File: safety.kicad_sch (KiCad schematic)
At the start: 23 parts, among them J5 Screw_Terminal_01x02, J7 Screw_Terminal_01x02, Q4 BSS138, SW1 SW_Push, SW2 SW_DIP_x03, SW3 SW_Push, U11 74LVC2G08, U16 74LVC1G175, U17 74HC123, Y2 SG-3031CM

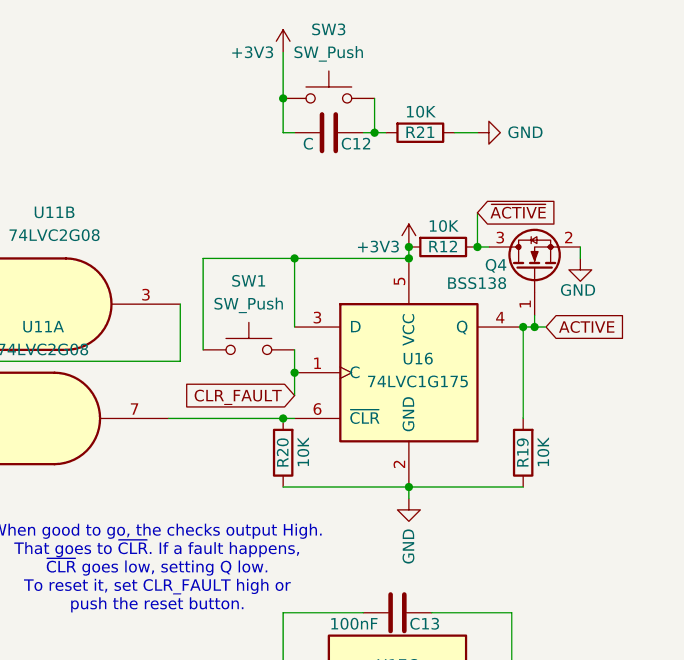
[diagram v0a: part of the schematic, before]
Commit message: Started on design, minor touch ups on schematic
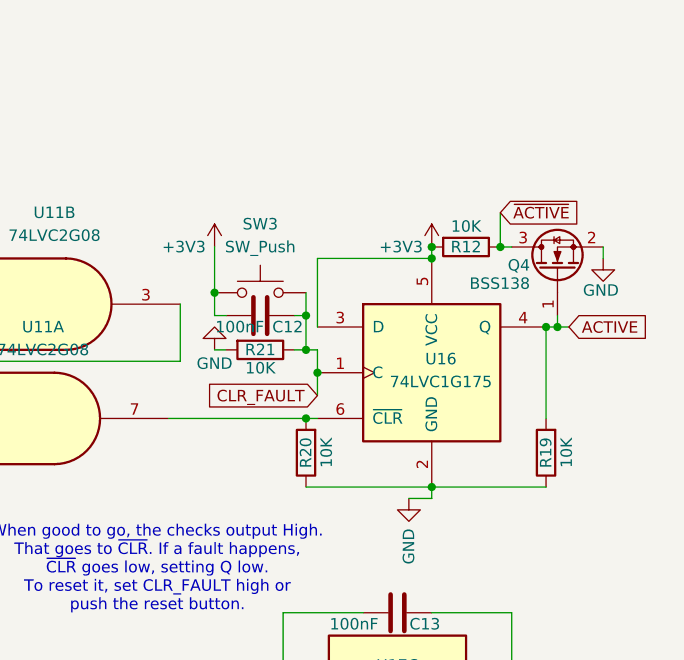
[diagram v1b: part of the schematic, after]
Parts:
- removed SW1: SW_Push, Button_Switch_SMD:SW_Push_1P1T_NO_CK_KMR2, symbol Switch:SW_Push
- C10, C11, C13, C14: footprint (none) -> Capacitor_SMD:C_0201_0603Metric_Pad0.64x0.40mm_HandSolder
- C12: value C -> 100nF; footprint (none) -> Capacitor_SMD:C_0201_0603Metric_Pad0.64x0.40mm_HandSolder
- R12, R15, R16, R19, R20, R21: footprint Resistor_SMD:R_0805_2012Metric_Pad1.20x1.40mm_HandSolder -> Resistor_SMD:R_0603_1608Metric_Pad0.98x0.95mm_HandSolder
- R17, R18: footprint (none) -> Resistor_SMD:R_0603_1608Metric_Pad0.98x0.95mm_HandSolder
- U11: footprint (none) -> Package_SO:VSSOP-8_2.3x2mm_P0.5mm
- U17: footprint (none) -> Package_SO:SOP-16_4.4x10.4mm_P1.27mm
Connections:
- net CLR_FAULT: now also C12.1, R21.1, SW3.2
- net GND: now also R21.2; no longer R21.1
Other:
- moved on the sheet: C12, Q4, R12, R19, R20, R21, SW3, U16
